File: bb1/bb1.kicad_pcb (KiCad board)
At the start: 4 copper layers, 101 x 56 mm, 101 parts, among them CON1 SD_Card, J1 USB-MICRO-B-SHIELDED, P1 PWR+CAN, P10 SPI_DBG, P11 CONN_01X02, P12 CONN_01X02, P13 CONN_01X02, P2 WIFI_DBG, P3 CONN_01X08, P4 USB_POWER, P5 NMEA_RX, P6 CORTEX_DEBUG, P7 NMEA_TX, P8 BATTERIES, P9 SHUNT, Q1 MMBT3904, SW1 RESET, SW2 PROGRAM, SW3 SW_PUSH, U1 TL2575, U10 MCP2562, U11 SN75C3222E, U12 INA219, U13 BMP280, U14 MPL3115A2, U2 WIFI_RGB, U3 ESP-13-WROOM-02, U4 N2K_RGB, U5 NMEA_RGB, U6 ILI9341_LCD_Breakout, U7 LP38691, U8 MK20DX256VLH7, U9 MKL02Z32VFG4, X1 CRYSTAL_SMD, Y2 32kHz

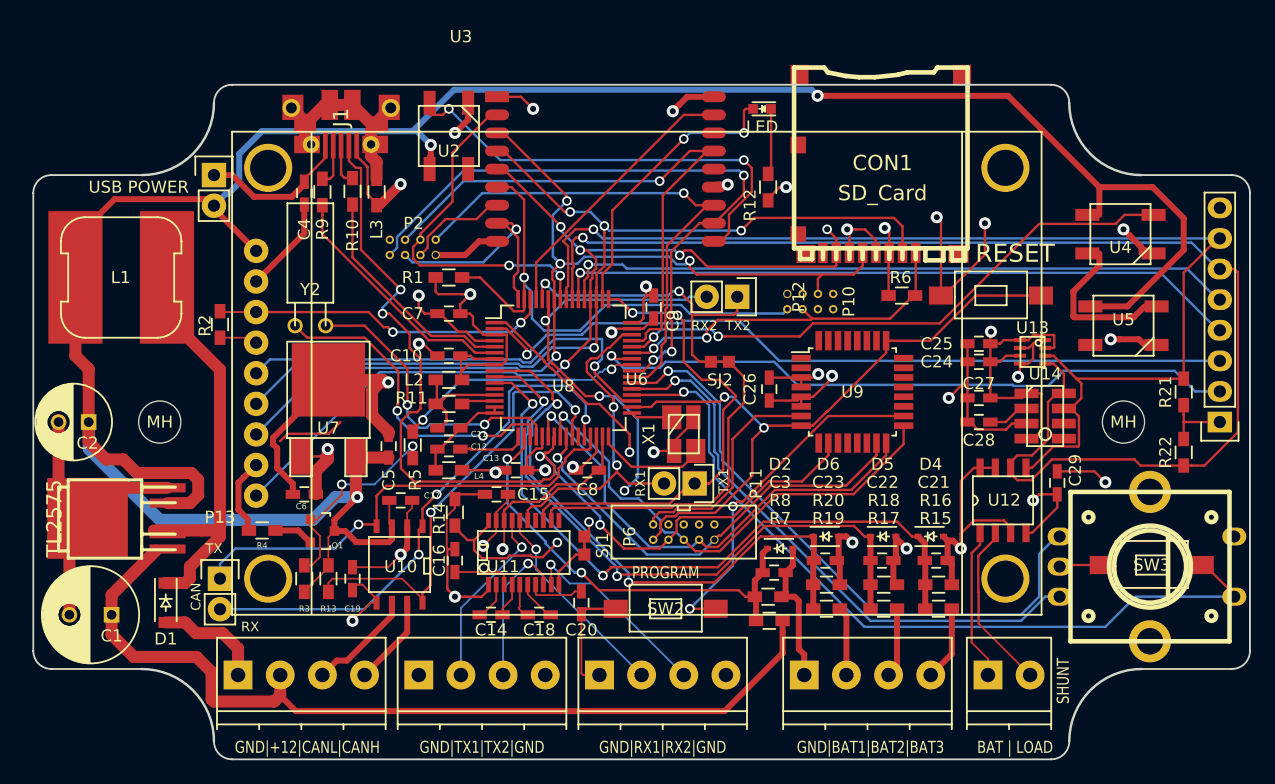
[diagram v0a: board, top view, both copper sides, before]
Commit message: Continued work on the PCB. Lots of footprint work.
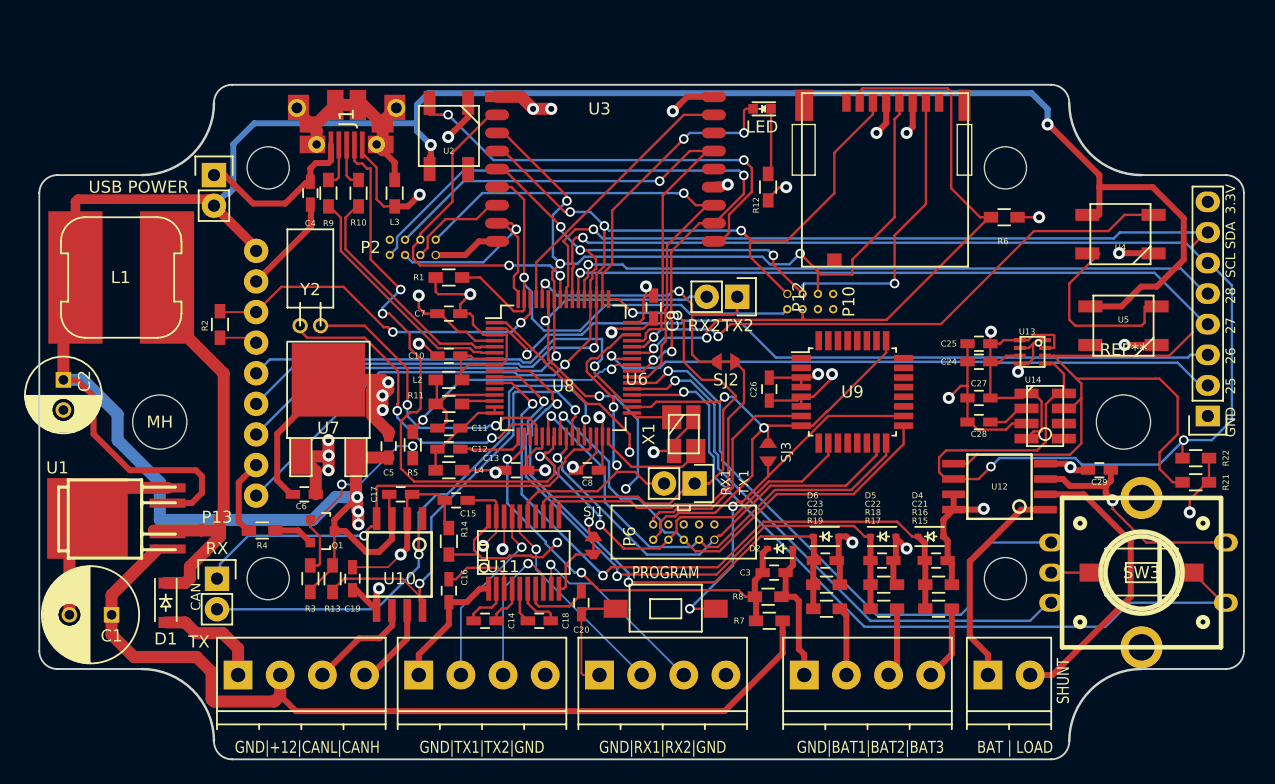
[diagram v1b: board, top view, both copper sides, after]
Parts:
- removed the MH at (127.0, 102.0)
- removed the MH at (47.0, 102.0)
- removed SW2: PROGRAM, bb:SWITCH_SMD_3x6
- added G***: LOGO, bb:BLUECOCONUT-LOGO_45mm, B.Cu at (111.7, 98.5)
- added MH: MountingHole_4-5mm, Mounting_Holes:MountingHole_4-5mm, F.Cu at (47.0, 102.0)
- added REF**: Symbol_OSHW-Logo_SilkScreen_BIG, Symbols:Symbol_OSHW-Logo_SilkScreen_BIG, B.Cu at (69.8, 77.5)
- added REF**: MountingHole_4-5mm, Mounting_Holes:MountingHole_4-5mm, F.Cu at (127.0, 102.0)
- added SJ3: SOLDER_JUMPER, bb:SolderJumper, F.Cu at (97.5, 104.5)
- CON1: value SD_Card -> MICROSD; footprint w_conn_misc:microsd_socket -> bb:DM3CS-SF
- SW1: value RESET -> PROGRAM
- U1: value TL2575 -> U1
- U10: footprint SMD_Packages:SOIC-8-N -> gsg-modules:SOIC8-208
- U11: footprint SMD_Packages:SSOP-20 -> bb:SSOP-20-HandSoldering
- U12: footprint bb:INA219 -> gsg-modules:SOIC8-208
- Y2: footprint Crystals:Crystal_Watch -> bb:Crystal_Watch_6mm
- moved SW1 37.5 mm to (89.0, 117.5)
- moved R6 10.7 mm to (117.1, 85.0), turned to 180 degrees
- moved R21 7.57 mm to (133.0, 107.0), turned to 180 degrees
- moved C2 4.08 mm to (39.0, 98.5), turned to 270 degrees
- moved C29 3.65 mm to (125.0, 106.0), turned to 0 degrees
- moved C15 3.39 mm to (71.6, 108.5)
- moved C16 2.55 mm to (71.0, 116.0), turned to 270 degrees
- moved R14 2.45 mm to (71.0, 111.9)
- moved L3 1.50 mm to (66.5, 83.0)
- moved CON1 1.37 mm to (107.2, 81.9)
- moved U12 1.17 mm to (116.7, 107.4), turned to 180 degrees
- moved P3 1.12 mm to (134.0, 101.5)
- moved R22 1.11 mm to (133.0, 105.0), turned to 180 degrees
- moved SW3 1.05 mm to (128.5, 114.5)
- moved E1 0.86 mm to (128.5, 114.5)
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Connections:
- CON1 pad 1: /Teensy/15/A1 -> Net-(CON1-Pad1)
- CON1 pad 2: /Teensy/11 -> /Teensy/15/A1
- CON1 pad 3: +3V3 -> /Teensy/11
- CON1 pad 4: GND -> +3V3
- P3 pad 1: +3V3 -> GND
- P3 pad 8: GND -> +3V3
- SJ1 pad 1: Net-(SJ1-Pad1) -> /Teensy/7
- SJ2 pad 2: Net-(SJ2-Pad2) -> /Teensy/8
- SW1 pad 1: /Teensy/RESET -> Net-(SJ3-Pad1)
- U11 pad 10: Net-(SJ1-Pad1) -> /Teensy/7
- U11 pad 12: Net-(SJ2-Pad2) -> /Teensy/8
- U9 pad 18: Net-(SW2-Pad1) -> Net-(SJ3-Pad1)
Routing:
- net Net-(SJ3-Pad1): track 0.00 -> 30.7 mm, vias 0 -> 2
- net /Teensy/8: track 26.2 -> 55.7 mm
- net Net-(SW2-Pad1): track 29.4 -> 0.00 mm, vias 2 -> 0
- net Net-(SJ2-Pad2): track 27.7 -> 0.00 mm
- net /Teensy/15/A1: track 30.9 -> 57.0 mm
- net GND: track 270.5 -> 246.2 mm
- net /Teensy/30: track 98.2 -> 121.4 mm
- net +5V: track 209.4 -> 231.7 mm, vias 3 -> 5
- net /Teensy/14/A0: track 79.9 -> 93.8 mm
- net /Teensy/12: track 83.4 -> 96.6 mm
- net /Teensy/RESET: track 55.8 -> 42.9 mm
- net /Teensy/29: track 109.0 -> 120.9 mm, vias 1 -> 3
- net Net-(P9-Pad2): track 14.2 -> 24.3 mm
- net /Teensy/7: track 42.4 -> 48.9 mm
- net (no net): track 5.65 -> 0.00 mm
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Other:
- board size 101 x 56 mm -> 100 x 56 mm
- board text added: "25"
- board text added: "26"
- board text added: "27"
- board text added: "28"
- board text added: "3.3V"
- board text added: "Blue Nexus v0.1 Copyright Thomas Sarlandie - 2015"
- board text added: "GND"
- board text added: "SCL"
- board text added: "SDA"
- board text removed: "BB1 v0.1 Open Source Hardware Copyright Thomas Sarlandie - 2015"
- board text removed: "RESET"
